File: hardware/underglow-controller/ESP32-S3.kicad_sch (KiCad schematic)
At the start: 39 parts, among them J101 CONSOLE, SW101 SW_Push, SW102 SW_Push, U101 ESP32-S3R2, U102 W25Q128JVS, Y101 40MHZ

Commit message: V5 Rev B Hardware release
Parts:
- TP101, TP102, TP103, TP104: now left out of the parts list
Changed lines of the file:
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@@
   )
   (symbol (lib_id "Connector:TestPoint") (at 228.6 21.59 270) (unit 1)
-    (in_bom yes) (on_board yes) (fields_autoplaced)
+    (in_bom no) (on_board yes) (fields_autoplaced)
     (property "Reference" "TP101" (id 0) (at 233.68 20.3199 90)
       (effects (font (size 1.27 1.27)) (justify left))
@@
   )
   (symbol (lib_id "Connector:TestPoint") (at 228.6 34.29 270) (unit 1)
-    (in_bom yes) (on_board yes) (fields_autoplaced)
+    (in_bom no) (on_board yes) (fields_autoplaced)
     (property "Reference" "TP103" (id 0) (at 233.68 33.0199 90)
       (effects (font (size 1.27 1.27)) (justify left))
@@
   )
   (symbol (lib_id "Connector:TestPoint") (at 228.6 40.64 270) (unit 1)
-    (in_bom yes) (on_board yes) (fields_autoplaced)
+    (in_bom no) (on_board yes) (fields_autoplaced)
     (property "Reference" "TP104" (id 0) (at 233.68 39.3699 90)
       (effects (font (size 1.27 1.27)) (justify left))
@@
   )
   (symbol (lib_id "Connector:TestPoint") (at 228.6 27.94 270) (unit 1)
-    (in_bom yes) (on_board yes) (fields_autoplaced)
+    (in_bom no) (on_board yes) (fields_autoplaced)
     (property "Reference" "TP102" (id 0) (at 233.68 26.6699 90)
       (effects (font (size 1.27 1.27)) (justify left))

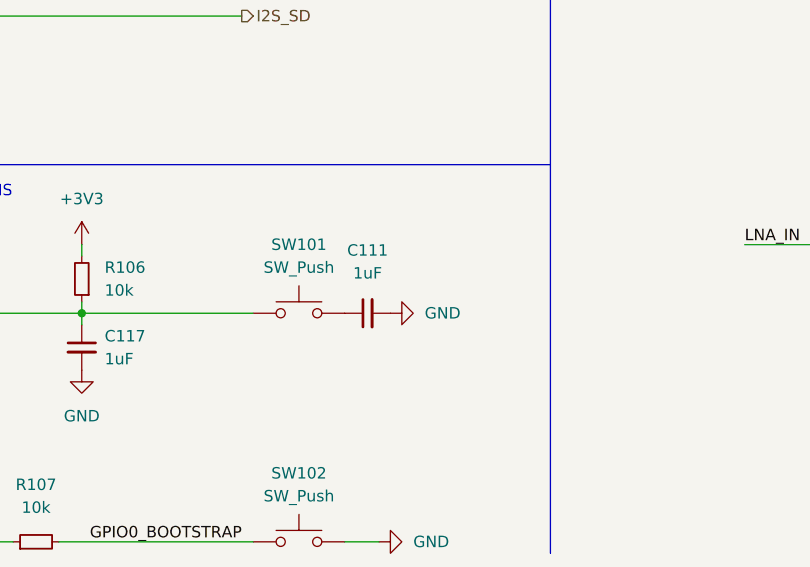
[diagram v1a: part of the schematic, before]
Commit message: hw updates based on latest boards
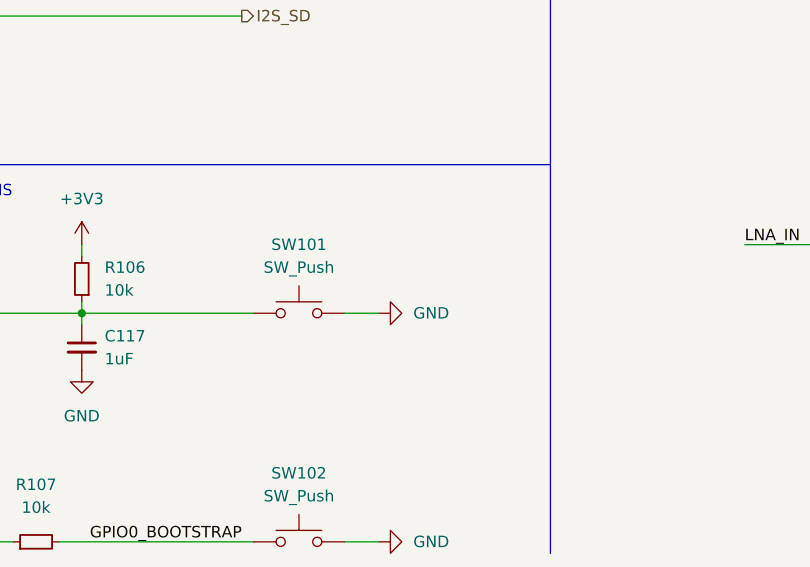
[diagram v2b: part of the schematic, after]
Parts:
- removed C111: 1uF, Capacitor_SMD:C_0402_1005Metric, symbol Device:C_Small
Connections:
- net GND: now also SW101.2
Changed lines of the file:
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@@
+    (stroke (width 0) (type default) (color 0 0 0 0))
+  )
+  (wire (pts (xy 154.94 139.7) (xy 158.75 139.7))
     (stroke (width 0) (type default) (color 0 0 0 0))
   )
@@
     )
     (pin "1")
-  )
-  (symbol (lib_id "Device:C_Small") (at 157.48 139.7 90) (unit 1)
-    (in_bom yes) (on_board yes) (fields_autoplaced)
-    (property "Reference" "C111" (id 0) (at 157.4863 132.715 90))
-    (property "Value" "1uF" (id 1) (at 157.4863 135.255 90))
-    (property "Footprint" "Capacitor_SMD:C_0402_1005Metric" (id 2) (at 157.48 139.7 0)
-      (effects (font (size 1.27 1.27)) hide)
-    )
-    (property "Datasheet" "~" (id 3) (at 157.48 139.7 0)
-      (effects (font (size 1.27 1.27)) hide)
-    )
-    (property "Description" "CAP CER 1UF 4V X7T 0402" (id 4) (at 157.48 139.7 0)
-      (effects (font (size 1.27 1.27)) hide)
-    )
-    (property "MPN" "CGA2B1X7T0G105M050BC" (id 5) (at 157.48 139.7 0)
-      (effects (font (size 1.27 1.27)) hide)
-    )
-    (pin "1")
-    (pin "2")
   )
   (symbol (lib_id "power:GND") (at 158.75 191.77 90) (unit 1)
@@
     (pin "2")
   )
-  (symbol (lib_id "power:GND") (at 160.02 139.7 90) (unit 1)
-    (in_bom yes) (on_board yes) (fields_autoplaced)
-    (property "Reference" "#PWR039" (id 0) (at 166.37 139.7 0)
-      (effects (font (size 1.27 1.27)) hide)
-    )
-    (property "Value" "GND" (id 1) (at 163.83 139.6999 90)
+  (symbol (lib_id "power:GND") (at 158.75 139.7 90) (unit 1)
+    (in_bom yes) (on_board yes) (fields_autoplaced)
+    (property "Reference" "#PWR039" (id 0) (at 165.1 139.7 0)
+      (effects (font (size 1.27 1.27)) hide)
+    )
+    (property "Value" "GND" (id 1) (at 162.56 139.6999 90)
       (effects (font (size 1.27 1.27)) (justify right))
     )
-    (property "Footprint" "" (id 2) (at 160.02 139.7 0)
-      (effects (font (size 1.27 1.27)) hide)
-    )
-    (property "Datasheet" "" (id 3) (at 160.02 139.7 0)
-      (effects (font (size 1.27 1.27)) hide)
-    )
+    (property "Footprint" "" (id 2) (at 158.75 139.7 0)
+      (effects (font (size 1.27 1.27)) hide)
+    )
+    (property "Datasheet" "" (id 3) (at 158.75 139.7 0)
+      (effects (font (size 1.27 1.27)) hide)
+    )
